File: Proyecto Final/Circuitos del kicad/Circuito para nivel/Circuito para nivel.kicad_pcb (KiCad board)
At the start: 2 copper layers, 49.5 x 35 mm, 16 parts, among them Q1 2N3904, Q2 2N3904, Q3 2N3904, Q4 2N3904

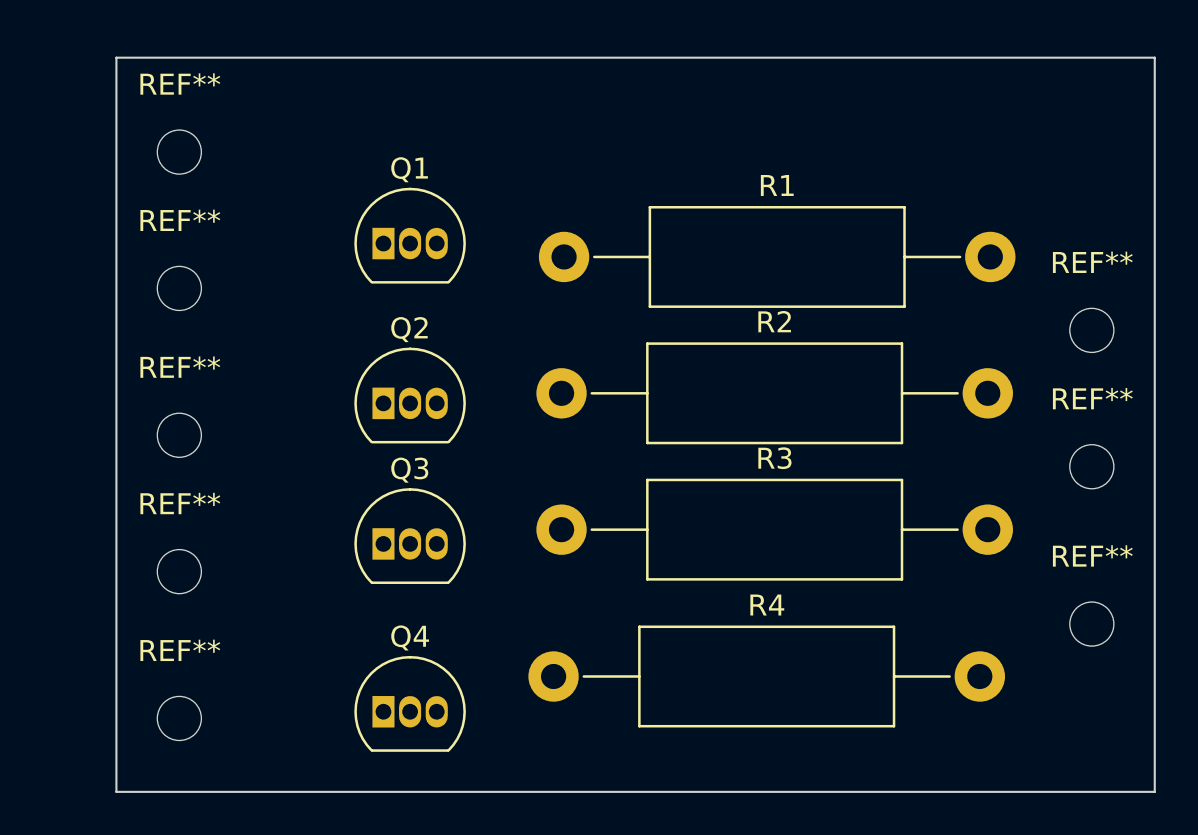
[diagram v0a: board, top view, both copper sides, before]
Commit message: ño
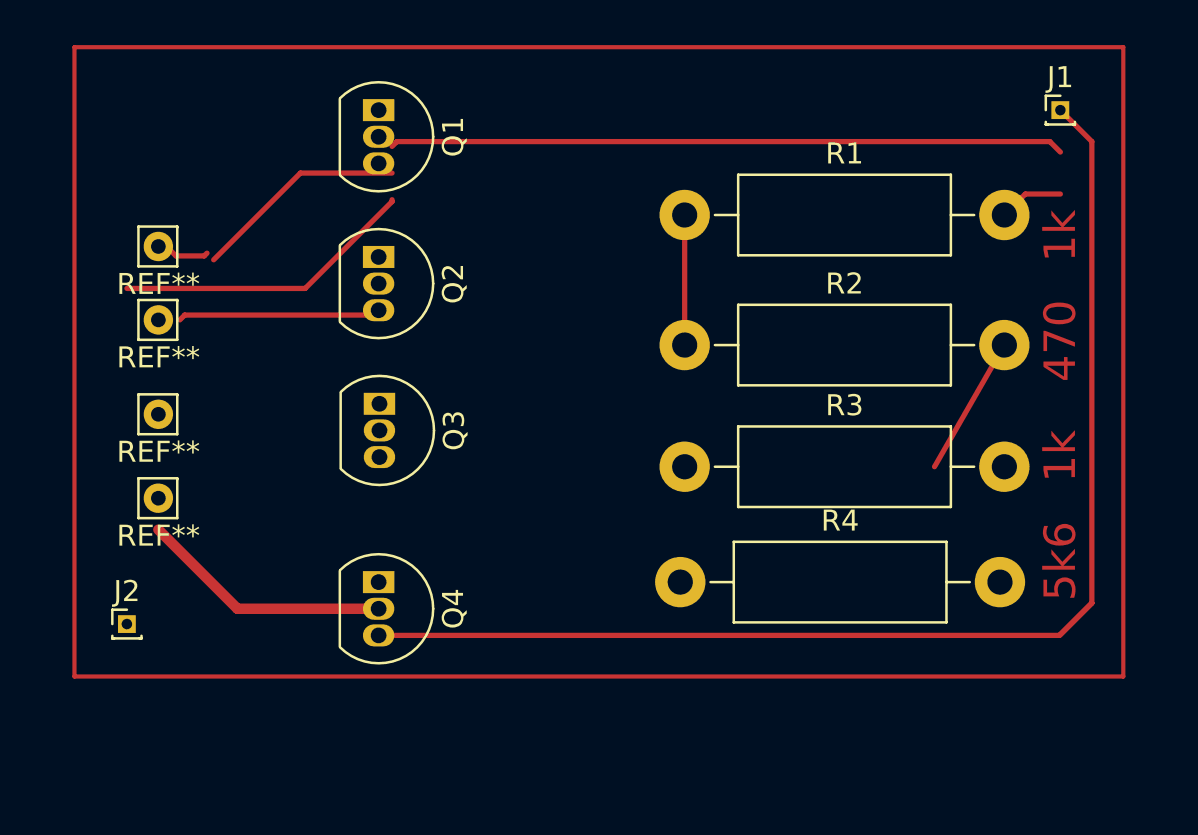
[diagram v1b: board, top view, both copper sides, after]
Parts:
- removed the REF** at (121.5, 87.0)
- removed the REF** at (165.0, 89.5)
- removed the REF** at (121.5, 94.0)
- removed the REF** at (121.5, 80.5)
- removed the REF** at (165.0, 82.0)
- removed the REF** at (121.5, 67.0)
- removed the REF** at (121.5, 73.5)
- removed the REF** at (165.0, 75.5)
- added J1: Conn_01x05, Connector_PinHeader_1.00mm:PinHeader_1x01_P1.00mm_Vertical, F.Cu at (163.5, 65.0)
- added J2: Conn_01x03, Connector_PinHeader_1.00mm:PinHeader_1x01_P1.00mm_Vertical, F.Cu at (119.0, 89.5)
- added REF**: Pin_D0.7mm_L6.5mm_W1.8mm_FlatFork, Connector_Pin:Pin_D0.7mm_L6.5mm_W1.8mm_FlatFork, F.Cu at (120.5, 71.5)
- added REF**: Pin_D0.7mm_L6.5mm_W1.8mm_FlatFork, Connector_Pin:Pin_D0.7mm_L6.5mm_W1.8mm_FlatFork, F.Cu at (120.5, 75.0)
- added REF**: Pin_D0.7mm_L6.5mm_W1.8mm_FlatFork, Connector_Pin:Pin_D0.7mm_L6.5mm_W1.8mm_FlatFork, F.Cu at (120.5, 83.5)
- added REF**: Pin_D0.7mm_L6.5mm_W1.8mm_FlatFork, Connector_Pin:Pin_D0.7mm_L6.5mm_W1.8mm_FlatFork, F.Cu at (120.5, 79.5)
- R1, R2, R3, R4: footprint Resistor_THT:R_Axial_DIN0414_L11.9mm_D4.5mm_P20.32mm_Horizontal -> Resistor_THT:R_Axial_DIN0411_L9.9mm_D3.6mm_P15.24mm_Horizontal
- moved R4 7.53 mm to (145.4, 87.5)
- moved Q2 6.98 mm to (131.0, 72.0), turned to -90 degrees
- moved Q3 6.68 mm to (131.0, 79.0), turned to -90 degrees
- moved R3 6.59 mm to (145.6, 82.0)
- moved Q1 6.36 mm to (131.0, 65.0), turned to -90 degrees
- moved R2 6.30 mm to (145.6, 76.2)
- moved Q4 6.18 mm to (131.0, 87.5), turned to -90 degrees
- moved R1 6.09 mm to (145.6, 70.0)
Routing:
- net VCC: track 0.00 -> 95.4 mm
- net level 100%: track 0.00 -> 32.2 mm
- net level 25%: track 0.00 -> 12.1 mm
- net Net-(Q2-Pad1): track 0.00 -> 6.69 mm
- net Datos para Arduino: track 0.00 -> 6.40 mm
- net GND: track 0.00 -> 3.08 mm
- net (no net): track 0.00 -> 2.56 mm
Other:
- board outline removed
- board text added: "1k"
- board text added: "470"
- board text added: "5k6"

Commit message: ñe
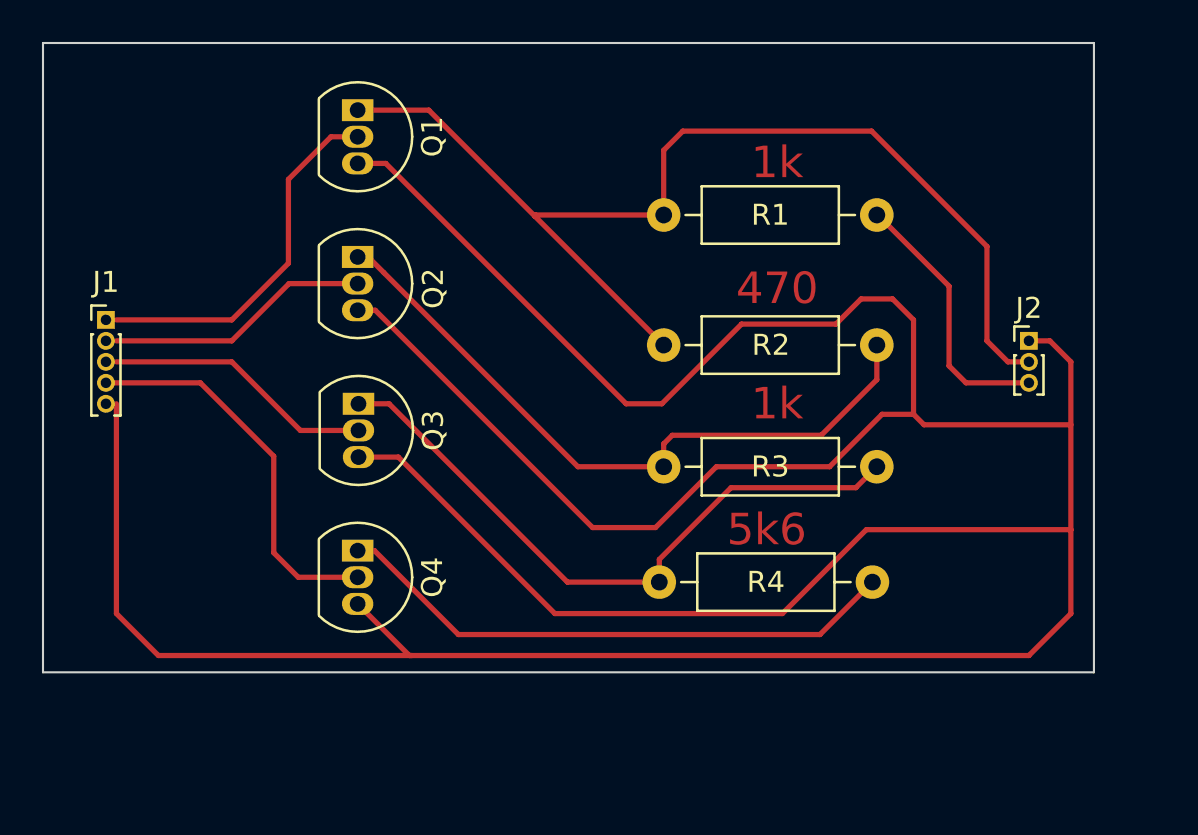
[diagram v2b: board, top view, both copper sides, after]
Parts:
- removed REF** (x4): Pin_D0.7mm_L6.5mm_W1.8mm_FlatFork, Connector_Pin:Pin_D0.7mm_L6.5mm_W1.8mm_FlatFork
- J1: footprint Connector_PinHeader_1.00mm:PinHeader_1x01_P1.00mm_Vertical -> Connector_PinHeader_1.00mm:PinHeader_1x05_P1.00mm_Vertical
- J2: footprint Connector_PinHeader_1.00mm:PinHeader_1x01_P1.00mm_Vertical -> Connector_PinHeader_1.00mm:PinHeader_1x03_P1.00mm_Vertical
- R1, R2, R3, R4: footprint Resistor_THT:R_Axial_DIN0411_L9.9mm_D3.6mm_P15.24mm_Horizontal -> Resistor_THT:R_Axial_DIN0207_L6.3mm_D2.5mm_P10.16mm_Horizontal
- moved J1 46.6 mm to (118.0, 75.0)
- moved J2 45.1 mm to (162.0, 76.0)
- moved Q4 1.80 mm to (130.0, 86.0)
- moved Q1 1.00 mm to (130.0, 65.0)
- moved Q2 1.00 mm to (130.0, 72.0)
- moved Q3 1.00 mm to (130.0, 79.0)
- moved R1 1.00 mm to (144.6, 70.0)
- moved R2 1.00 mm to (144.6, 76.2)
- moved R3 1.00 mm to (144.6, 82.0)
- moved R4 1.00 mm to (144.4, 87.5)
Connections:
- J1 pad 1: VCC -> level 100%
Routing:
- net VCC: track 95.4 -> 192.9 mm
- net Datos para Arduino: track 6.40 -> 53.5 mm
- net Net-(Q3-Pad1): track 0.00 -> 31.1 mm
- net Net-(Q4-Pad1): track 0.00 -> 27.2 mm
- net Net-(Q2-Pad1): track 6.69 -> 32.9 mm
- net level 100%: track 32.2 -> 17.5 mm
- net level 50%: track 0.00 -> 12.9 mm
- net level 75%: track 0.00 -> 12.6 mm
- net GND: track 3.08 -> 12.8 mm
- net level 25%: track 12.1 -> 18.5 mm
- net (no net): track 2.56 -> 0.00 mm
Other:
- board outline added: 50.1 x 30 mm
- board text added: "Así estaría bien, pero no se si se tiene que espejar para que se imprima bien la placa"
